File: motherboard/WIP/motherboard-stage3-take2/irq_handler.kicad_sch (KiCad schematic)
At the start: 16 parts, among them U16 74HCT02, U17 74HCT148, U18 74HCT148, U19 74HCT574, U20 74HCT00, U21 74HCT574, U22 74HCT85

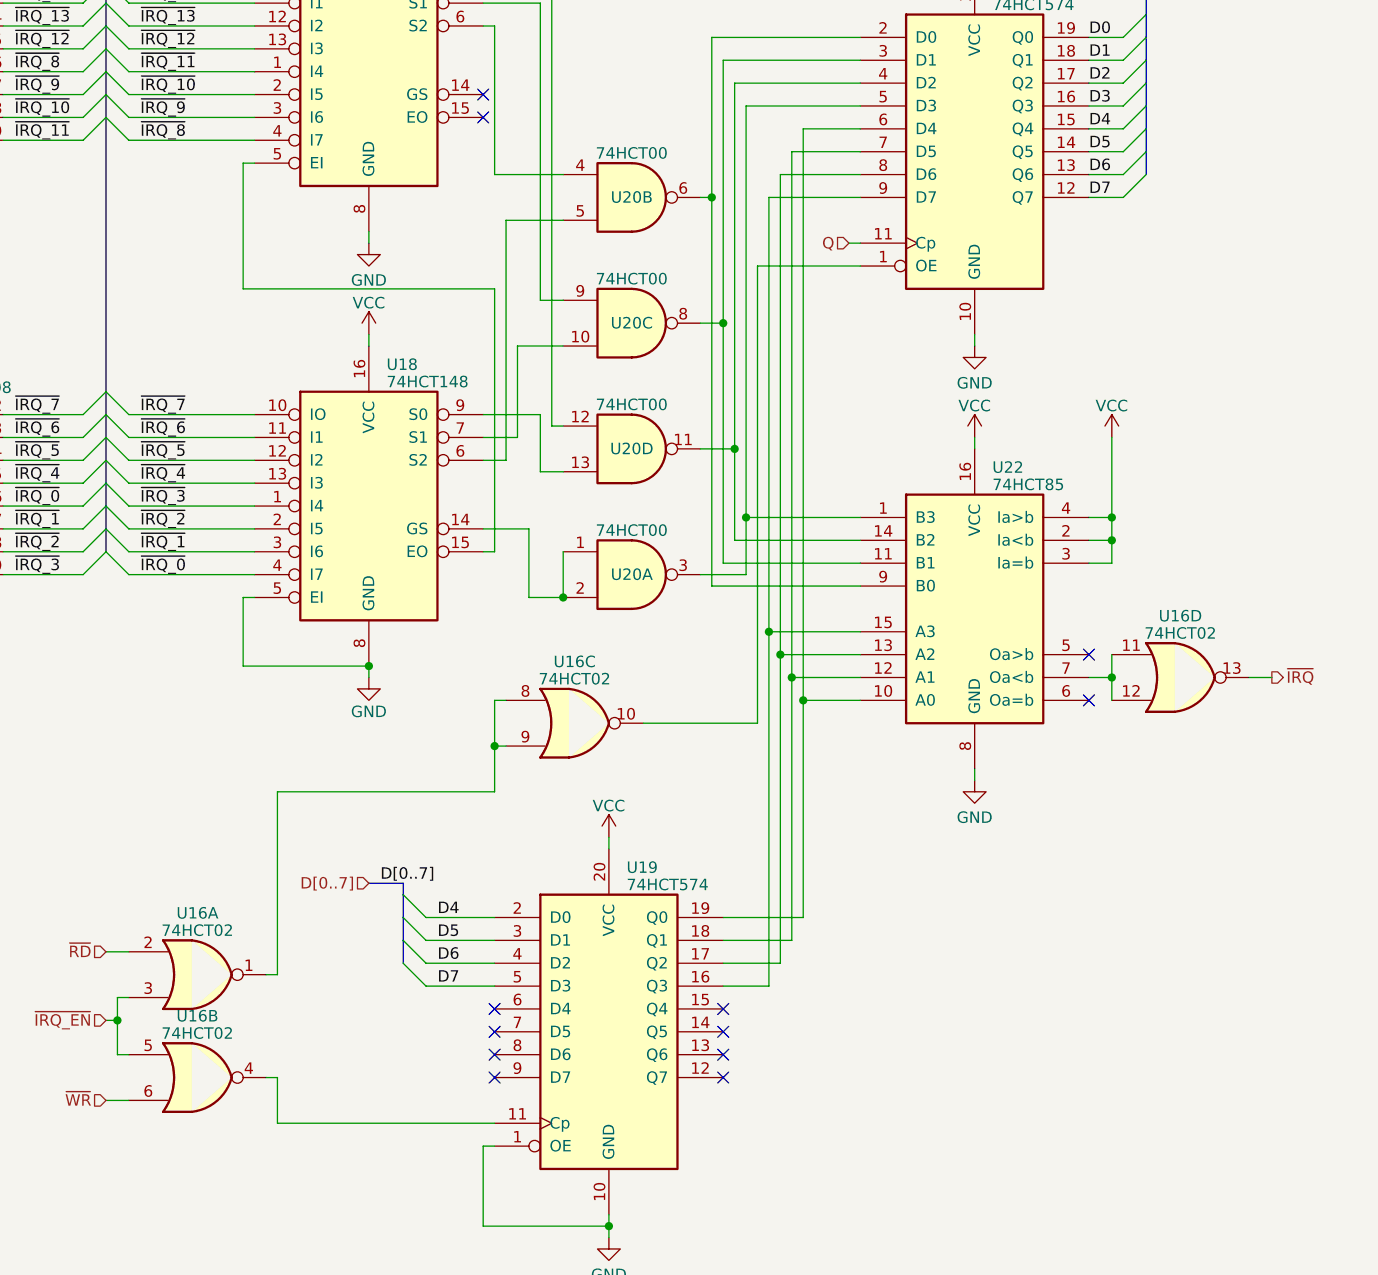
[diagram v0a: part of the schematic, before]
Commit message: Updates
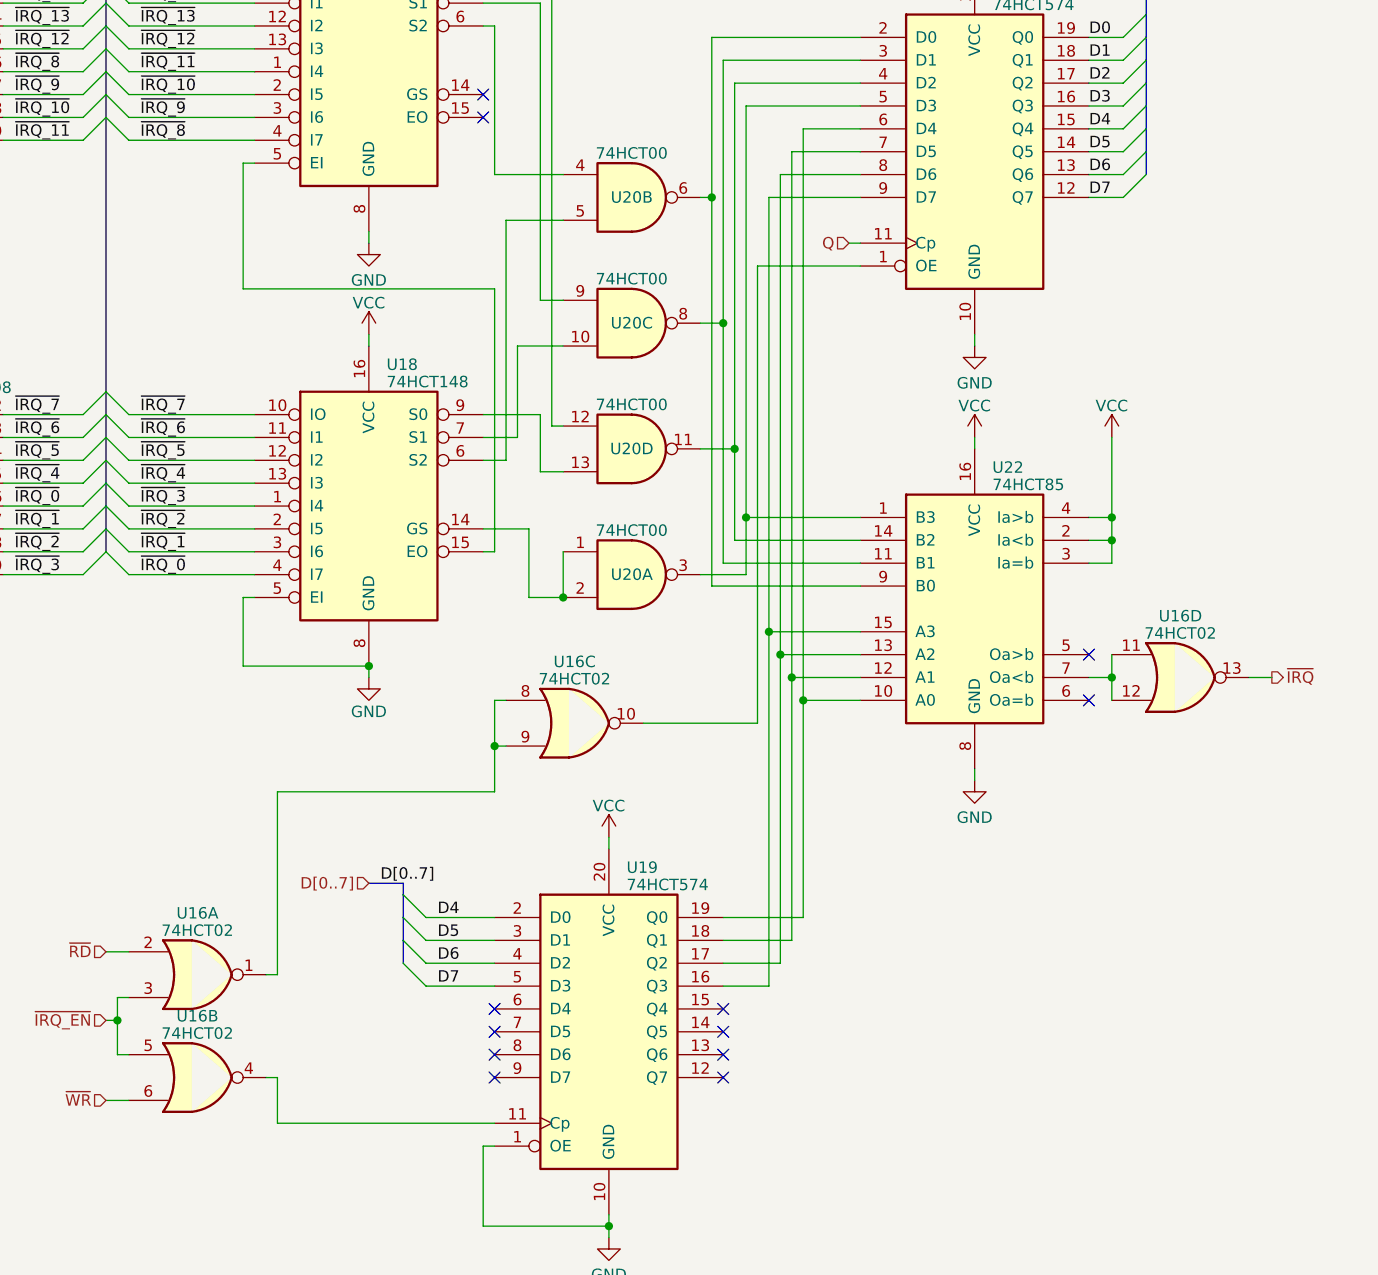
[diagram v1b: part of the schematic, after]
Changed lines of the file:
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@@
 (kicad_sch
-	(version 20231120)
+	(version 20250114)
 	(generator "eeschema")
-	(generator_version "8.0")
+	(generator_version "9.0")
 	(paper "A4")
 	(title_block
@@
 	(label "~{IRQ_9}"
 		(at 34.29 62.23 0)
-		(fields_autoplaced yes)
 		(effects
 			(font
@@
 	(label "~{IRQ_4}"
 		(at 34.29 105.41 0)
-		(fields_autoplaced yes)
 		(effects
 			(font
@@
 	(label "~{IRQ_6}"
 		(at 48.26 100.33 0)
-		(fields_autoplaced yes)
 		(effects
 			(font
@@
 	(label "D1"
 		(at 153.67 58.42 0)
-		(fields_autoplaced yes)
 		(effects
 			(font
@@
 	(label "~{IRQ_2}"
 		(at 34.29 113.03 0)
-		(fields_autoplaced yes)
 		(effects
 			(font
@@
 	(label "D7"
 		(at 81.28 161.29 0)
-		(fields_autoplaced yes)
 		(effects
 			(font
@@
 	(label "D7"
 		(at 153.67 73.66 0)
-		(fields_autoplaced yes)
 		(effects
 			(font
@@
 	(label "~{IRQ_5}"
 		(at 34.29 102.87 0)
-		(fields_autoplaced yes)
 		(effects
 			(font
@@
 	(label "D4"
 		(at 153.67 66.04 0)
-		(fields_autoplaced yes)
 		(effects
 			(font
@@
 	(label "~{IRQ_14}"
 		(at 48.26 52.07 0)
-		(fields_autoplaced yes)
 		(effects
 			(font
@@
 	(label "~{IRQ_3}"
 		(at 48.26 107.95 0)
-		(fields_autoplaced yes)
 		(effects
 			(font
@@
 	(label "~{IRQ_13}"
 		(at 48.26 54.61 0)
-		(fields_autoplaced yes)
 		(effects
 			(font
@@
 	(label "D6"
 		(at 81.28 158.75 0)
-		(fields_autoplaced yes)
 		(effects
 			(font
@@
 	(label "D[0..7]"
 		(at 162.56 46.99 0)
-		(fields_autoplaced yes)
 		(effects
 			(font
@@
 	(label "~{IRQ_4}"
 		(at 48.26 105.41 0)
-		(fields_autoplaced yes)
 		(effects
 			(font
@@
 	(label "D5"
 		(at 81.28 156.21 0)
-		(fields_autoplaced yes)
 		(effects
 			(font
@@
 	(label "~{IRQ_9}"
 		(at 48.26 64.77 0)
-		(fields_autoplaced yes)
 		(effects
 			(font
@@
 	(label "~{IRQ_10}"
 		(at 48.26 62.23 0)
-		(fields_autoplaced yes)
 		(effects
 			(font
@@
 	(label "~{IRQ_7}"
 		(at 48.26 97.79 0)
-		(fields_autoplaced yes)
 		(effects
 			(font
@@
 	(label "D6"
 		(at 153.67 71.12 0)
-		(fields_autoplaced yes)
 		(effects
 			(font
@@
 	(label "~{IRQ_12}"
 		(at 34.29 57.15 0)
-		(fields_autoplaced yes)
 		(effects
 			(font
@@
 	(label "~{IRQ_5}"
 		(at 48.26 102.87 0)
-		(fields_autoplaced yes)
 		(effects
 			(font
@@
 	(label "~{IRQ_7}"
 		(at 34.29 97.79 0)
-		(fields_autoplaced yes)
 		(effects
 			(font
@@
 	(label "~{IRQ_11}"
 		(at 48.26 59.69 0)
-		(fields_autoplaced yes)
 		(effects
 			(font
@@
 	(label "~{IRQ_13}"
 		(at 34.29 54.61 0)
-		(fields_autoplaced yes)
 		(effects
 			(font
@@
 	(label "~{IRQ_11}"
 		(at 34.29 67.31 0)
-		(fields_autoplaced yes)
 		(effects
 			(font
@@
 	(label "~{IRQ_8}"
 		(at 34.29 59.69 0)
-		(fields_autoplaced yes)
 		(effects
 			(font
@@
 	(label "~{IRQ_1}"
 		(at 48.26 113.03 0)
-		(fields_autoplaced yes)
 		(effects
 			(font
@@
 	(label "~{IRQ_1}"
 		(at 34.29 110.49 0)
-		(fields_autoplaced yes)
 		(effects
 			(font
@@
 	(label "~{IRQ_[0..15]}"
 		(at 35.56 39.37 0)
-		(fields_autoplaced yes)
 		(effects
 			(font
@@
 	(label "~{IRQ_0}"
 		(at 48.26 115.57 0)
-		(fields_autoplaced yes)
 		(effects
 			(font
@@
 	(label "D[0..7]"
 		(at 74.93 149.86 0)
-		(fields_autoplaced yes)
 		(effects
 			(font
@@
 	(label "D2"
 		(at 153.67 60.96 0)
-		(fields_autoplaced yes)
 		(effects
 			(font
@@
 	(label "D5"
 		(at 153.67 68.58 0)
-		(fields_autoplaced yes)
 		(effects
 			(font
@@
 	(label "~{IRQ_12}"
 		(at 48.26 57.15 0)
-		(fields_autoplaced yes)
 		(effects
 			(font
@@
 	(label "D0"
 		(at 153.67 55.88 0)
-		(fields_autoplaced yes)
 		(effects
 			(font
@@
 	(label "~{IRQ_8}"
 		(at 48.26 67.31 0)
-		(fields_autoplaced yes)
 		(effects
 			(font
@@
 	(label "~{IRQ_2}"
 		(at 48.26 110.49 0)
-		(fields_autoplaced yes)
 		(effects
 			(font
@@
 	(label "~{IRQ_0}"
 		(at 34.29 107.95 0)
-		(fields_autoplaced yes)
 		(effects
 			(font
@@
 	(label "~{IRQ_14}"
 		(at 34.29 52.07 0)
-		(fields_autoplaced yes)
 		(effects
 			(font
@@
 	(label "~{IRQ_3}"
 		(at 34.29 115.57 0)
-		(fields_autoplaced yes)
 		(effects
 			(font
@@
 	(label "~{IRQ_6}"
 		(at 34.29 100.33 0)
-		(fields_autoplaced yes)
 		(effects
 			(font
@@
 	(label "D3"
 		(at 153.67 63.5 0)
-		(fields_autoplaced yes)
 		(effects
 			(font
@@
 	(label "~{IRQ_10}"
 		(at 34.29 64.77 0)
-		(fields_autoplaced yes)
 		(effects
 			(font
@@
 	(label "D4"
 		(at 81.28 153.67 0)
-		(fields_autoplaced yes)
 		(effects
 			(font
@@
 		(shape output)
 		(at 173.99 127 0)
-		(fields_autoplaced yes)
 		(effects
 			(font
@@
 		(shape input)
 		(at 44.45 173.99 180)
-		(fields_autoplaced yes)
 		(effects
 			(font
@@
 		(shape input)
 		(at 127 78.74 180)
-		(fields_autoplaced yes)
 		(effects
 			(font
@@
 		(shape input)
 		(at 34.29 39.37 180)
-		(fields_autoplaced yes)
 		(effects
 			(font
@@
 		(shape input)
 		(at 73.66 149.86 180)
-		(fields_autoplaced yes)
 		(effects
 			(font
@@
 		(shape input)
 		(at 44.45 165.1 180)
-		(fields_autoplaced yes)
 		(effects
 			(font
@@
 		(shape input)
 		(at 44.45 157.48 180)
-		(fields_autoplaced yes)
 		(effects
 			(font
@@
 		(shape input)
 		(at 170.18 46.99 0)
-		(fields_autoplaced yes)
 		(effects
 			(font
